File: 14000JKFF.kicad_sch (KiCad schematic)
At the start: 33 parts, among them IC2 74AHC573PW,118, IC3 74LVC1G3157DW-7, IC35 SN74AHC1G04DBVR, IC6 74LVC1G3157DW-7

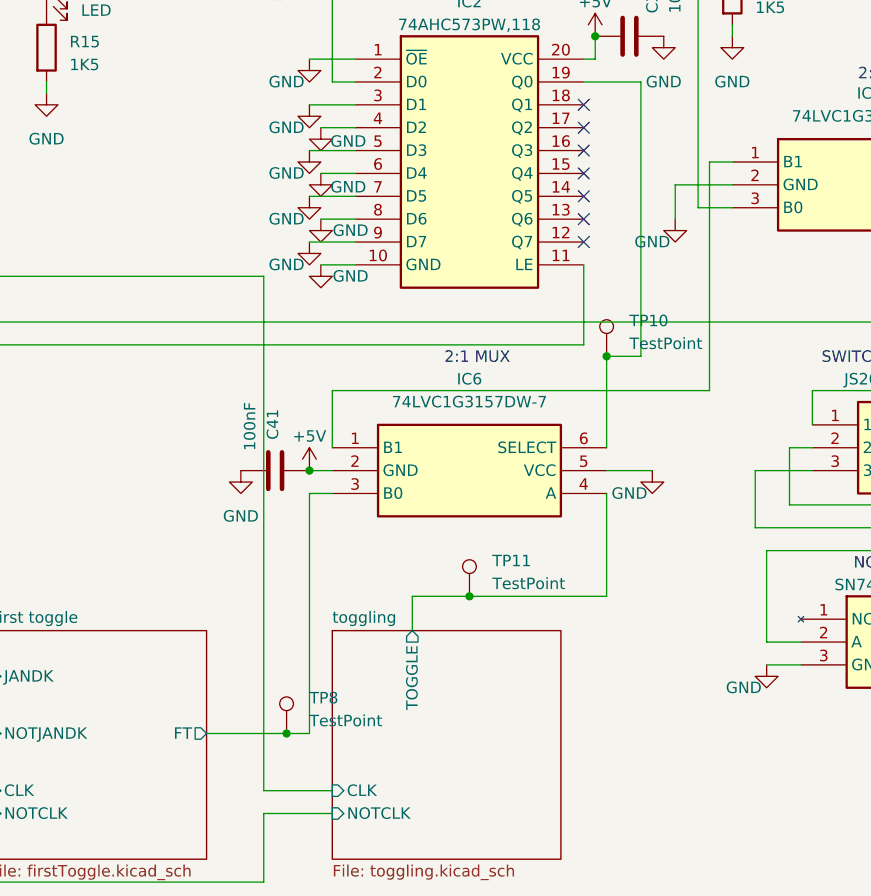
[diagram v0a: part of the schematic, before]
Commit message: Add files via upload
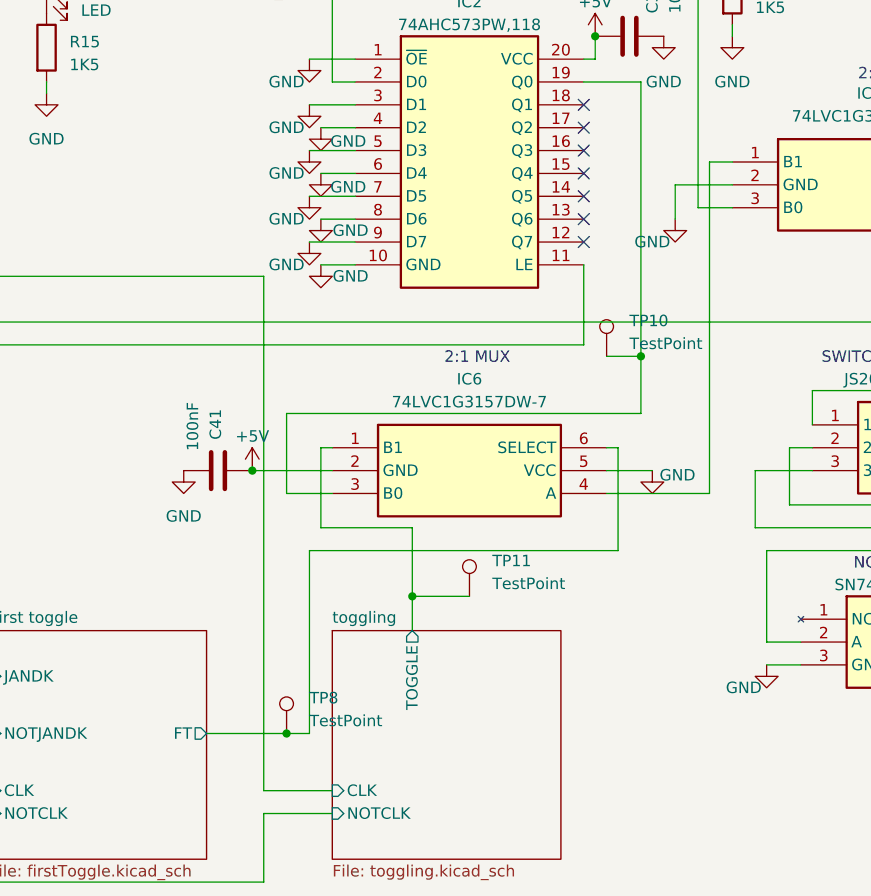
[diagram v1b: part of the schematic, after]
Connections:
- net First toggle/FT: now also IC6.6 (SELECT); no longer IC6.3 (B0)
- net toggling/TOGGLE: now also IC6.1 (B1); no longer IC6.4 (A)
- net at IC2.19 (Q0), TP10.1: now also IC6.3 (B0); no longer IC6.6 (SELECT)
- net at IC3.1 (B1): now also IC6.4 (A); no longer IC6.1 (B1)
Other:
- moved on the sheet: C41
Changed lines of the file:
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@@
 	)
 	(junction
-		(at 181.61 115.57)
+		(at 175.26 115.57)
 		(diameter 0)
 		(color 0 0 0 0)
@@
 	)
 	(junction
-		(at 213.36 67.31)
+		(at 193.04 129.54)
 		(diameter 0)
 		(color 0 0 0 0)
 	)
 	(junction
-		(at 77.47 48.26)
+		(at 213.36 67.31)
 		(diameter 0)
 		(color 0 0 0 0)
 	)
 	(junction
-		(at 179.07 144.78)
+		(at 77.47 48.26)
 		(diameter 0)
 		(color 0 0 0 0)
 	)
 	(junction
-		(at 139.7 153.67)
+		(at 179.07 144.78)
 		(diameter 0)
 		(color 0 0 0 0)
 	)
 	(junction
-		(at 214.63 102.87)
+		(at 139.7 153.67)
 		(diameter 0)
 		(color 0 0 0 0)
@@
 	)
 	(junction
-		(at 199.39 129.54)
+		(at 218.44 102.87)
 		(diameter 0)
 		(color 0 0 0 0)
@@
 	(wire
 		(pts
+			(xy 226.06 118.11) (xy 214.63 118.11)
+		)
+		(stroke
+			(width 0)
+			(type default)
+		)
+	)
+	(wire
+		(pts
 			(xy 139.7 161.29) (xy 176.53 161.29)
 		)
@@
 	(wire
 		(pts
-			(xy 260.35 113.03) (xy 257.81 113.03)
+			(xy 215.9 113.03) (xy 214.63 113.03)
 		)
 		(stroke
@@
 	(wire
 		(pts
-			(xy 133.35 99.06) (xy 133.35 138.43)
+			(xy 260.35 113.03) (xy 257.81 113.03)
 		)
 		(stroke
@@
 	(wire
 		(pts
-			(xy 77.47 74.93) (xy 87.63 74.93)
+			(xy 133.35 99.06) (xy 133.35 138.43)
 		)
 		(stroke
@@
 	(wire
 		(pts
-			(xy 182.88 82.55) (xy 186.69 82.55)
+			(xy 77.47 74.93) (xy 87.63 74.93)
 		)
 		(stroke
@@
 	(wire
 		(pts
-			(xy 212.09 72.39) (xy 218.44 72.39)
+			(xy 182.88 82.55) (xy 186.69 82.55)
 		)
 		(stroke
@@
 	(wire
 		(pts
-			(xy 222.25 83.82) (xy 228.6 83.82)
+			(xy 212.09 72.39) (xy 218.44 72.39)
 		)
 		(stroke
@@
 	(wire
 		(pts
-			(xy 81.28 80.01) (xy 81.28 153.67)
+			(xy 222.25 83.82) (xy 228.6 83.82)
 		)
 		(stroke
@@
 	(wire
 		(pts
-			(xy 102.87 101.6) (xy 128.27 101.6)
+			(xy 81.28 80.01) (xy 81.28 153.67)
 		)
 		(stroke
@@
 	(wire
 		(pts
-			(xy 184.15 113.03) (xy 184.15 106.68)
+			(xy 102.87 101.6) (xy 128.27 101.6)
 		)
 		(stroke
@@
 	(wire
 		(pts
-			(xy 184.15 106.68) (xy 226.06 106.68)
+			(xy 267.97 134.62) (xy 267.97 132.08)
 		)
 		(stroke
@@
 	(wire
 		(pts
-			(xy 267.97 134.62) (xy 267.97 132.08)
+			(xy 262.89 115.57) (xy 262.89 121.92)
 		)
 		(stroke
@@
 	(wire
 		(pts
-			(xy 262.89 115.57) (xy 262.89 121.92)
+			(xy 181.61 144.78) (xy 181.61 124.46)
 		)
 		(stroke
@@
 	(wire
 		(pts
-			(xy 181.61 118.11) (xy 184.15 118.11)
+			(xy 260.35 100.33) (xy 271.78 100.33)
 		)
 		(stroke
@@
 	(wire
 		(pts
-			(xy 260.35 100.33) (xy 271.78 100.33)
+			(xy 182.88 113.03) (xy 182.88 121.92)
 		)
 		(stroke
@@
 	(wire
 		(pts
-			(xy 214.63 129.54) (xy 214.63 118.11)
-		)
-		(stroke
-			(width 0)
-			(type default)
-		)
-	)
-	(wire
-		(pts
 			(xy 176.53 161.29) (xy 176.53 153.67)
 		)
@@
 	(wire
 		(pts
-			(xy 226.06 81.28) (xy 226.06 106.68)
+			(xy 226.06 81.28) (xy 226.06 118.11)
 		)
 		(stroke
@@
 	(wire
 		(pts
-			(xy 199.39 129.54) (xy 214.63 129.54)
+			(xy 181.61 124.46) (xy 215.9 124.46)
+		)
+		(stroke
+			(width 0)
+			(type default)
+		)
+	)
+	(wire
+		(pts
+			(xy 193.04 121.92) (xy 193.04 129.54)
 		)
 		(stroke
@@
 	(wire
 		(pts
-			(xy 181.61 115.57) (xy 184.15 115.57)
+			(xy 175.26 115.57) (xy 184.15 115.57)
 		)
 		(stroke
@@
 	(wire
 		(pts
+			(xy 179.07 109.22) (xy 218.44 109.22)
+		)
+		(stroke
+			(width 0)
+			(type default)
+		)
+	)
+	(wire
+		(pts
 			(xy 123.19 93.98) (xy 176.53 93.98)
 		)
@@
 	(wire
 		(pts
-			(xy 214.63 102.87) (xy 214.63 113.03)
+			(xy 181.61 74.93) (xy 186.69 74.93)
 		)
 		(stroke
@@
 	(wire
 		(pts
-			(xy 181.61 74.93) (xy 186.69 74.93)
+			(xy 260.35 119.38) (xy 260.35 113.03)
 		)
 		(stroke
@@
 	(wire
 		(pts
-			(xy 260.35 119.38) (xy 260.35 113.03)
+			(xy 184.15 50.8) (xy 180.34 50.8)
 		)
 		(stroke
@@
 	(wire
 		(pts
-			(xy 184.15 50.8) (xy 180.34 50.8)
+			(xy 262.89 121.92) (xy 231.14 121.92)
 		)
 		(stroke
@@
 	(wire
 		(pts
-			(xy 262.89 121.92) (xy 231.14 121.92)
+			(xy 215.9 124.46) (xy 215.9 113.03)
 		)
 		(stroke
@@
 	(wire
 		(pts
+			(xy 218.44 102.87) (xy 218.44 109.22)
+		)
+		(stroke
+			(width 0)
+			(type default)
+		)
+	)
+	(wire
+		(pts
+			(xy 184.15 113.03) (xy 182.88 113.03)
+		)
+		(stroke
+			(width 0)
+			(type default)
+		)
+	)
+	(wire
+		(pts
 			(xy 50.8 82.55) (xy 50.8 99.06)
 		)
@@
 	(wire
 		(pts
-			(xy 138.43 54.61) (xy 140.97 54.61)
+			(xy 182.88 121.92) (xy 193.04 121.92)
 		)
 		(stroke
@@
 	(wire
 		(pts
-			(xy 152.4 48.26) (xy 152.4 57.15)
+			(xy 138.43 54.61) (xy 140.97 54.61)
 		)
 		(stroke
@@
 	(wire
 		(pts
-			(xy 182.88 87.63) (xy 186.69 87.63)
+			(xy 152.4 48.26) (xy 152.4 57.15)
 		)
 		(stroke
@@
 	(wire
 		(pts
-			(xy 181.61 118.11) (xy 181.61 144.78)
+			(xy 182.88 87.63) (xy 186.69 87.63)
 		)
 		(stroke
@@
 	(wire
 		(pts
+			(xy 179.07 118.11) (xy 184.15 118.11)
+		)
+		(stroke
+			(width 0)
+			(type default)
+		)
+	)
+	(wire
+		(pts
 			(xy 77.47 48.26) (xy 92.71 48.26)
 		)
@@
 	(wire
 		(pts
+			(xy 179.07 109.22) (xy 179.07 118.11)
+		)
+		(stroke
+			(width 0)
+			(type default)
+		)
+	)
+	(wire
+		(pts
 			(xy 139.7 153.67) (xy 139.7 161.29)
 		)
@@
 	(symbol
 		(lib_id "power:+5V")
-		(at 181.61 115.57 0)
+		(at 175.26 115.57 0)
 		(unit 1)
 		(exclude_from_sim no)
@@
 		(dnp no)
 		(property "Reference" "#PWR0134"
-			(at 181.61 119.38 0)
+			(at 175.26 119.38 0)
 			(effects
 				(font
@@
 		)
 		(property "Value" "+5V"
-			(at 181.61 111.76 0)
+			(at 175.26 111.76 0)
 			(effects
 				(font
@@
 		)
 		(property "Footprint" ""
-			(at 181.61 115.57 0)
+			(at 175.26 115.57 0)
 			(effects
 				(font
@@
 		)
 		(property "Datasheet" ""
-			(at 181.61 115.57 0)
+			(at 175.26 115.57 0)
 			(effects
 				(font
@@
 		)
 		(property "Description" ""
-			(at 181.61 115.57 0)
+			(at 175.26 115.57 0)
 			(effects
 				(font
@@
 	(symbol
 		(lib_id "power:GND")
-		(at 173.99 115.57 0)
+		(at 167.64 115.57 0)
 		(unit 1)
 		(exclude_from_sim no)
@@
 		(fields_autoplaced yes)
 		(property "Reference" "#PWR0135"
-			(at 173.99 121.92 0)
+			(at 167.64 121.92 0)
 			(effects
 				(font
@@
 		)
 		(property "Value" "GND"
-			(at 173.99 120.65 0)
+			(at 167.64 120.65 0)
 			(effects
 				(font
@@
 		)
 		(property "Footprint" ""
-			(at 173.99 115.57 0)
+			(at 167.64 115.57 0)
 			(effects
 				(font
@@
 		)
 		(property "Datasheet" ""
-			(at 173.99 115.57 0)
+			(at 167.64 115.57 0)
 			(effects
 				(font
@@
 		)
 		(property "Description" ""
-			(at 173.99 115.57 0)
+			(at 167.64 115.57 0)
 			(effects
 				(font
@@
 	(symbol
 		(lib_id "Device:C")
-		(at 177.8 115.57 90)
+		(at 171.45 115.57 90)
 		(unit 1)
 		(exclude_from_sim no)
@@
 		(dnp no)
 		(property "Reference" "C41"
-			(at 177.546 108.712 0)
+			(at 171.196 108.712 0)
 			(effects
 				(font
@@
 		)
 		(property "Value" "100nF"
-			(at 175.006 107.95 0)
+			(at 168.656 107.95 0)
 			(effects
 				(font
@@
 		)
 		(property "Footprint" "Capacitor_SMD:C_1206_3216Metric"
-			(at 181.61 114.6048 0)
+			(at 175.26 114.6048 0)
 			(effects
 				(font
@@
 		)
 		(property "Datasheet" "~"
-			(at 177.8 115.57 0)
+			(at 171.45 115.57 0)
 			(effects
 				(font
@@
 		)
 		(property "Description" ""
-			(at 177.8 115.57 0)
+			(at 171.45 115.57 0)
 			(effects
 				(font
@@
 		)
 		(property "Value" "GND"
-			(at 217.17 118.11 0)
+			(at 222.504 116.078 0)
 			(effects
 				(font
